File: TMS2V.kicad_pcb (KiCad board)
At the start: 2 copper layers, 37 parts, among them J1 TMS9918A Socket, J3 RGB Out, J4 RGB Header, Q1 BC547, Q2 BC547, Q3 BC547, Q4 BC547, U1 V9938, U2 D41464, U3 D41464, U4 D41464, U5 D41464, Y1 24.47727 Mhz

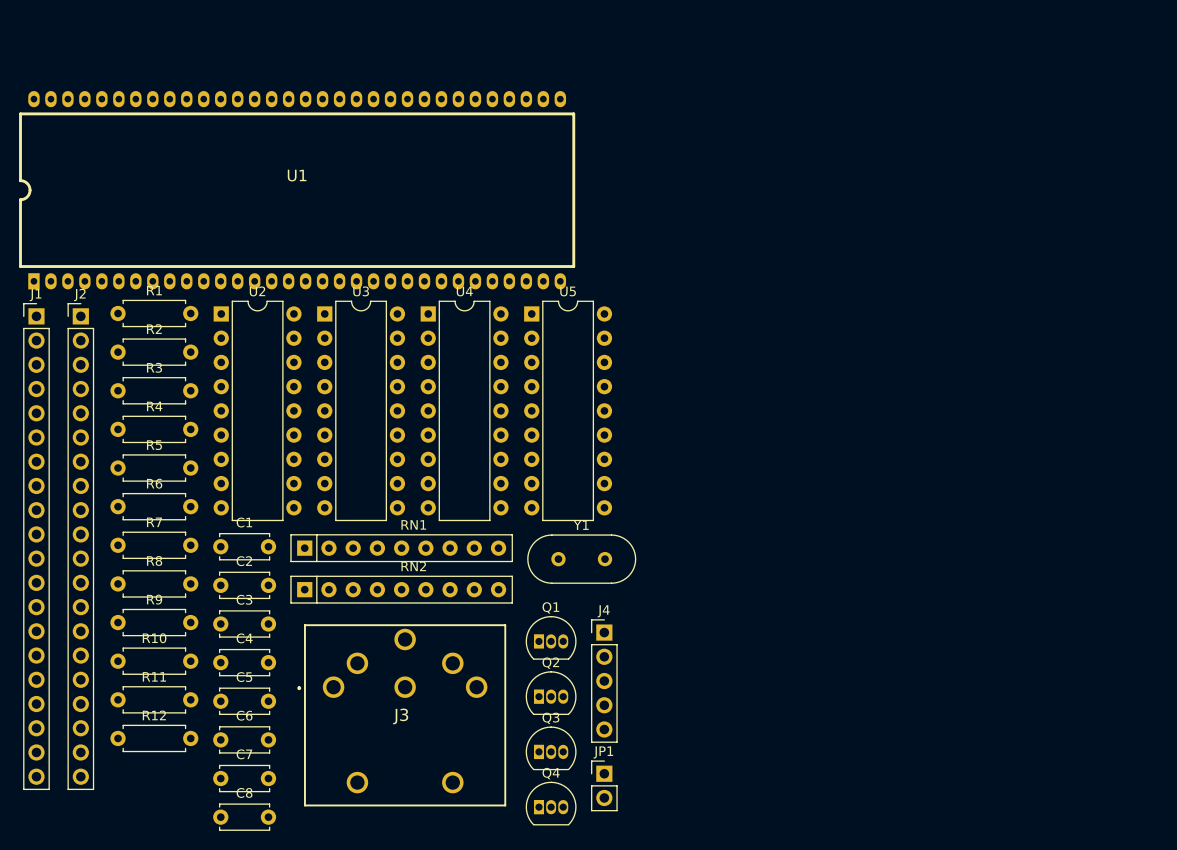
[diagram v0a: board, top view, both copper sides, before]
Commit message: Initial PCB layout
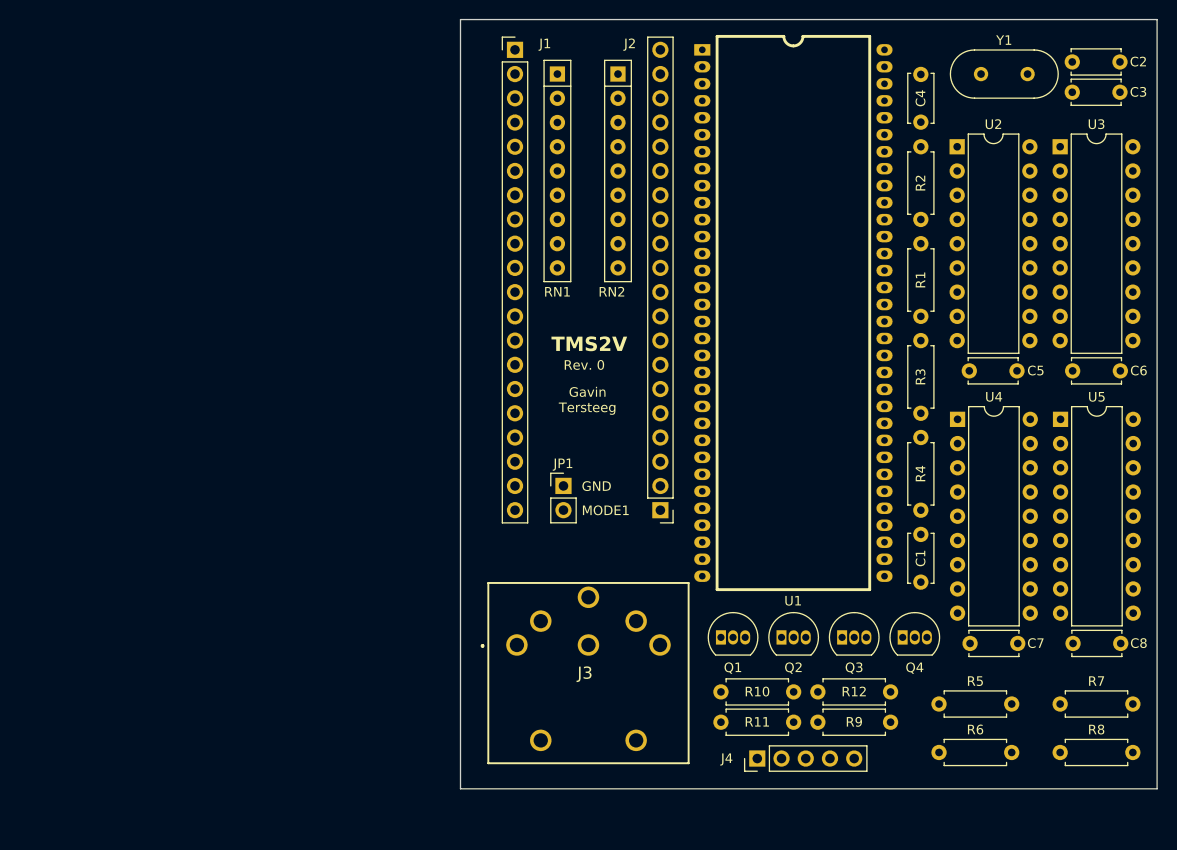
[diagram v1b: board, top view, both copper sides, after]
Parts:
- moved C3 109.5 mm to (186.0, 80.0), turned to 180 degrees
- moved C2 109.1 mm to (186.0, 76.8), turned to 180 degrees
- moved R8 100.3 mm to (179.7, 149.2)
- moved R7 100.2 mm to (179.7, 144.1)
- moved C6 97.3 mm to (181.0, 109.2)
- moved C4 92.7 mm to (165.1, 83.1), turned to 90 degrees
- moved C8 91.2 mm to (181.1, 137.8)
- moved R6 89.8 mm to (167.0, 149.2)
- moved R5 89.6 mm to (167.0, 144.1)
- moved R2 86.9 mm to (165.1, 85.7), turned to -90 degrees
- moved C5 85.8 mm to (170.2, 109.2)
- moved R4 84.6 mm to (165.1, 123.8), turned to 90 degrees
- moved R1 84.5 mm to (165.1, 95.9), turned to -90 degrees
- moved R3 84.2 mm to (165.1, 113.7), turned to 90 degrees
- moved C7 79.8 mm to (170.3, 137.8)
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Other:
- board outline added: 73 x 80.6 mm
- board text added: "GND"
- board text added: "Gavin Tersteeg"
- board text added: "MODE1"
- board text added: "Rev. 0"
- board text added: "TMS2V"
